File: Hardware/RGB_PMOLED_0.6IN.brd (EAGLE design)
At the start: 22.9 x 30.5 mm, 46 parts, among them Q1 310mA/60V/1.6Ω, U1 UG-6464TDDBG01, U2 AP3012, U3 3.3V, U4 TXB0104

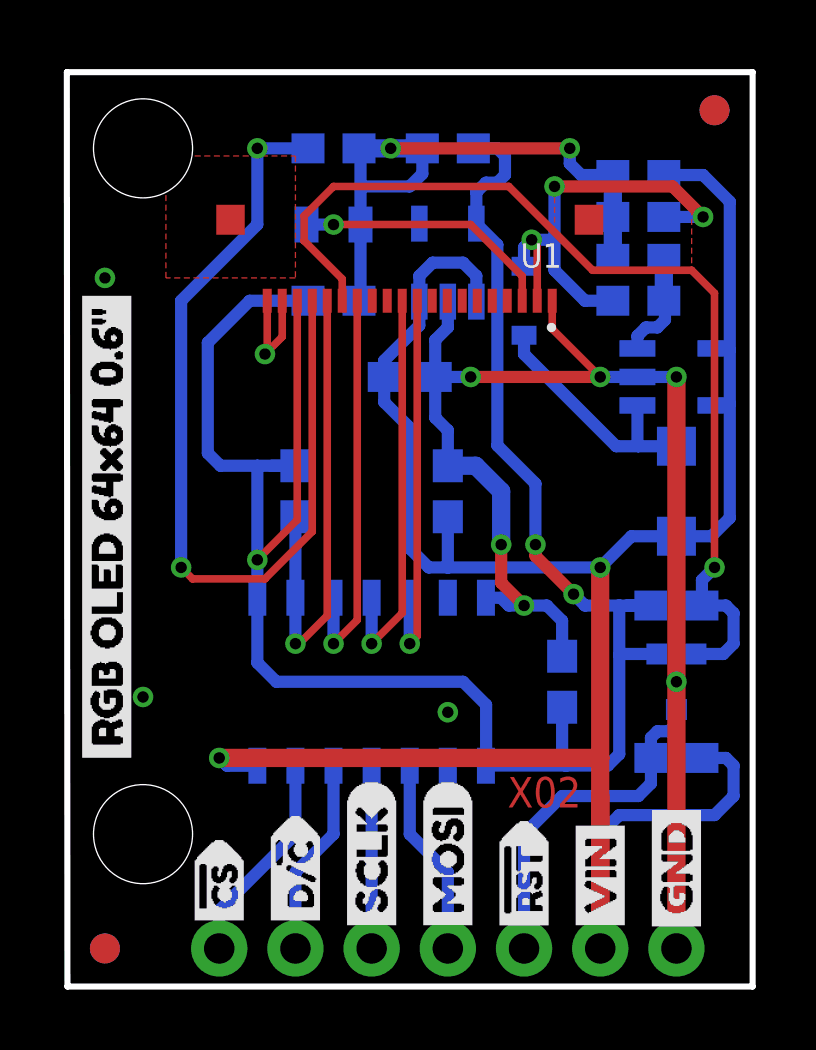
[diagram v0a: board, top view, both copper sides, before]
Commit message: Cleaned up documentation
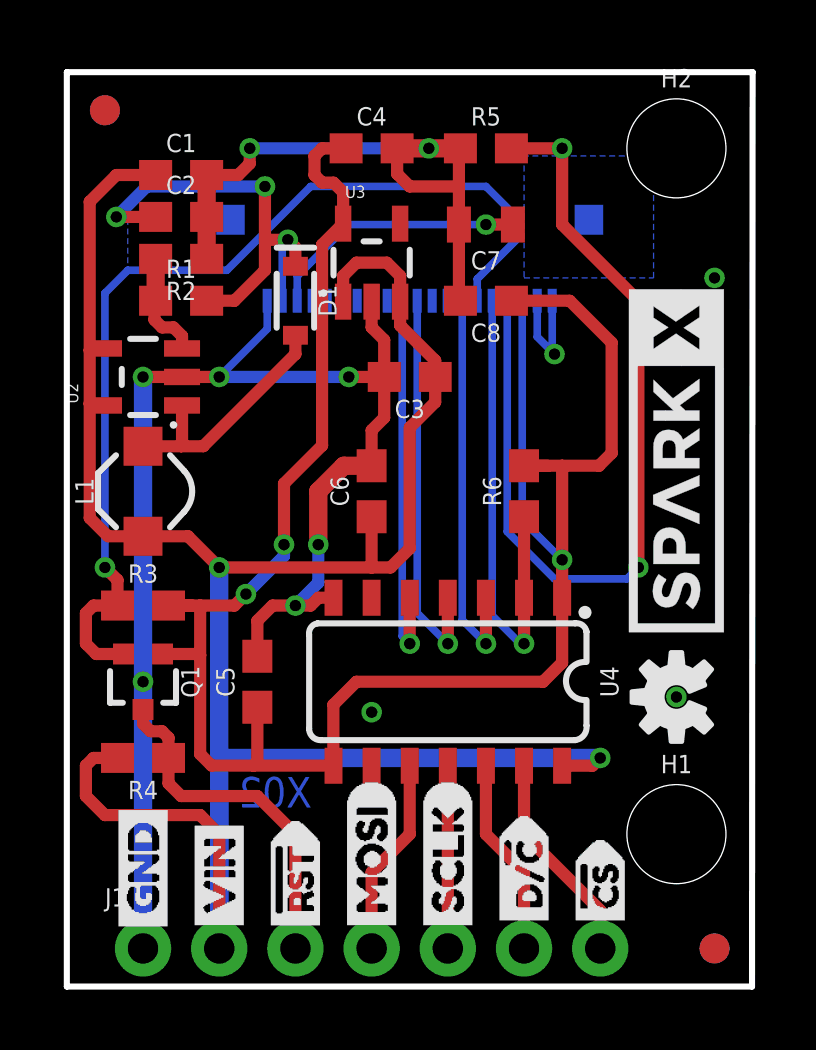
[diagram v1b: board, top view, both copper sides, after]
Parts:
- moved FRAME1 45.7 mm to (-11.4, -14.0), flipped to the top
- moved FD1 20.3 mm to (1.27, 29.2), flipped to the top
- moved FD2 20.3 mm to (21.6, 1.27), flipped to the top
- moved FD3 20.3 mm to (21.6, 1.27), flipped to the bottom
- moved FD4 20.3 mm to (1.27, 29.2), flipped to the bottom
- moved U$16 20.2 mm to (21.5, 7.11), flipped to the bottom
- moved H1 17.8 mm to (20.3, 5.08), flipped to the top
- moved H2 17.8 mm to (20.3, 27.9), flipped to the top
- moved J1 17.8 mm to (2.54, 1.27), flipped to the top
- moved L1 17.8 mm to (2.54, 16.5), flipped to the top
- moved LOGO1 17.8 mm to (20.3, 17.5), flipped to the top
- moved LOGO2 17.8 mm to (20.3, 9.65), flipped to the top
- moved Q1 17.8 mm to (2.54, 10.2), flipped to the top
- moved R3 17.8 mm to (2.54, 12.7), flipped to the top
- moved R4 17.8 mm to (2.54, 7.62), flipped to the top
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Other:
- outline, holes or cut-outs redrawn
